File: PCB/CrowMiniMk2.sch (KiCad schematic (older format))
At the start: 21 parts

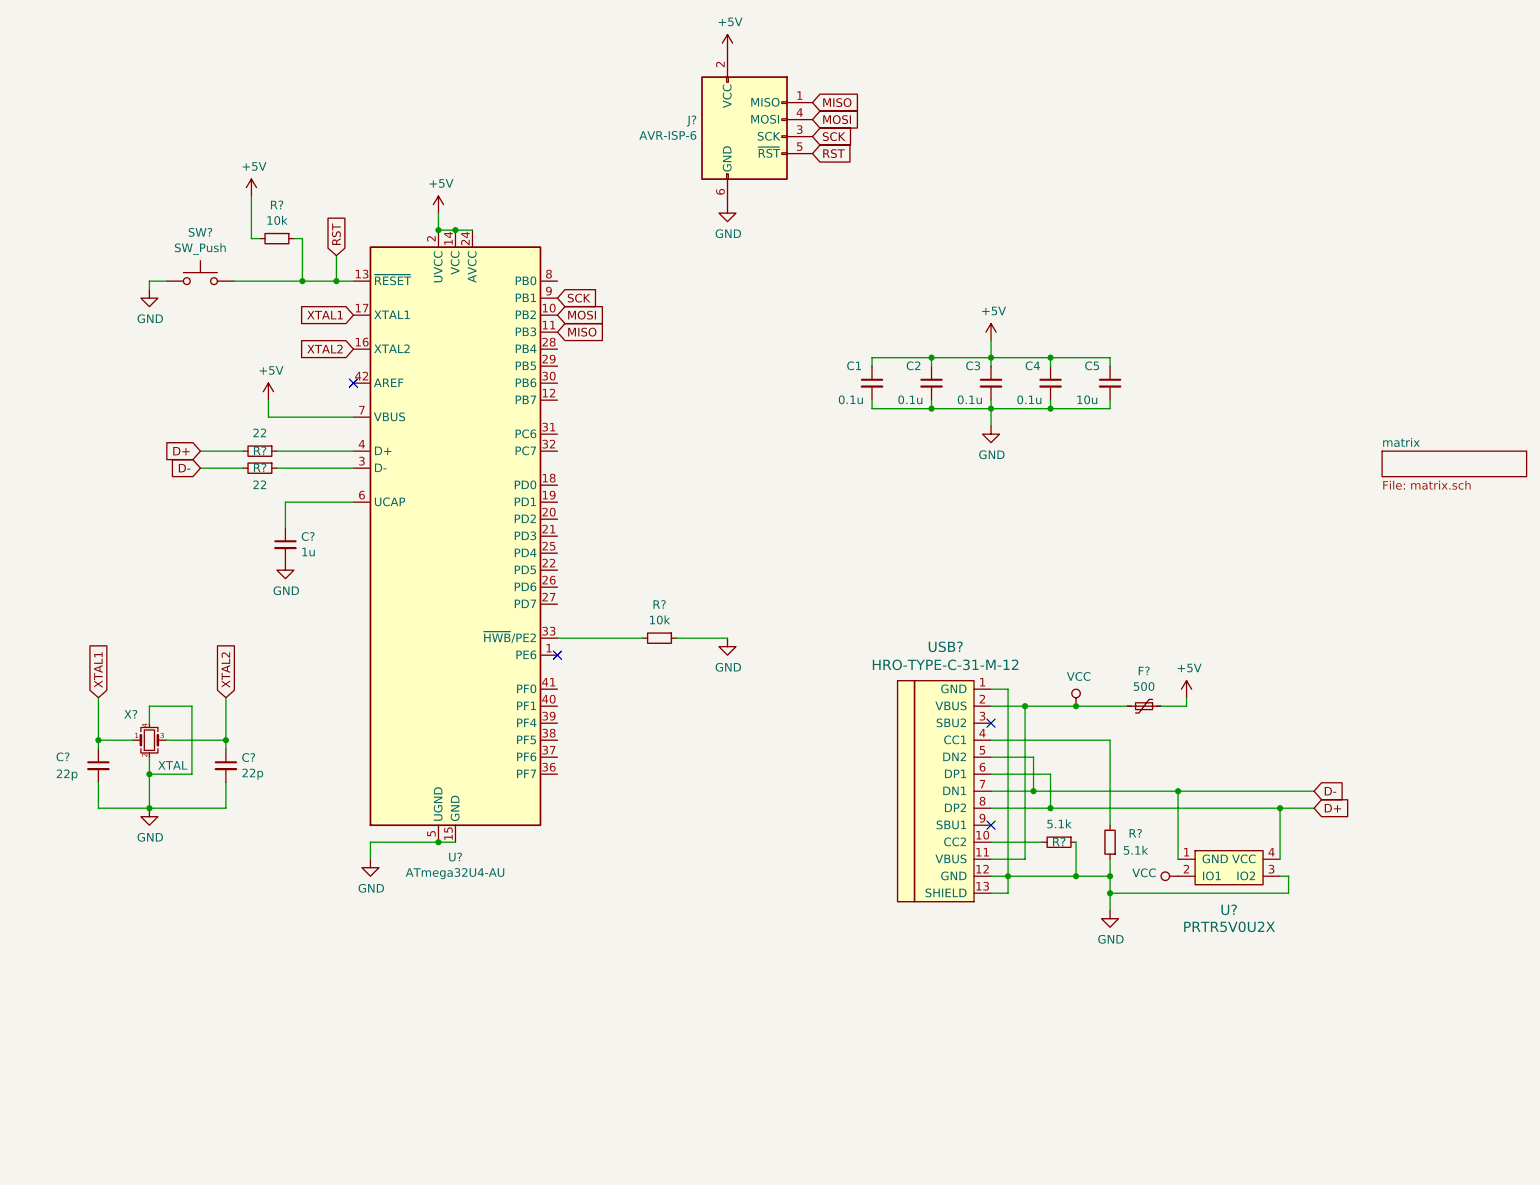
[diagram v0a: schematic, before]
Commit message: Sch Finish
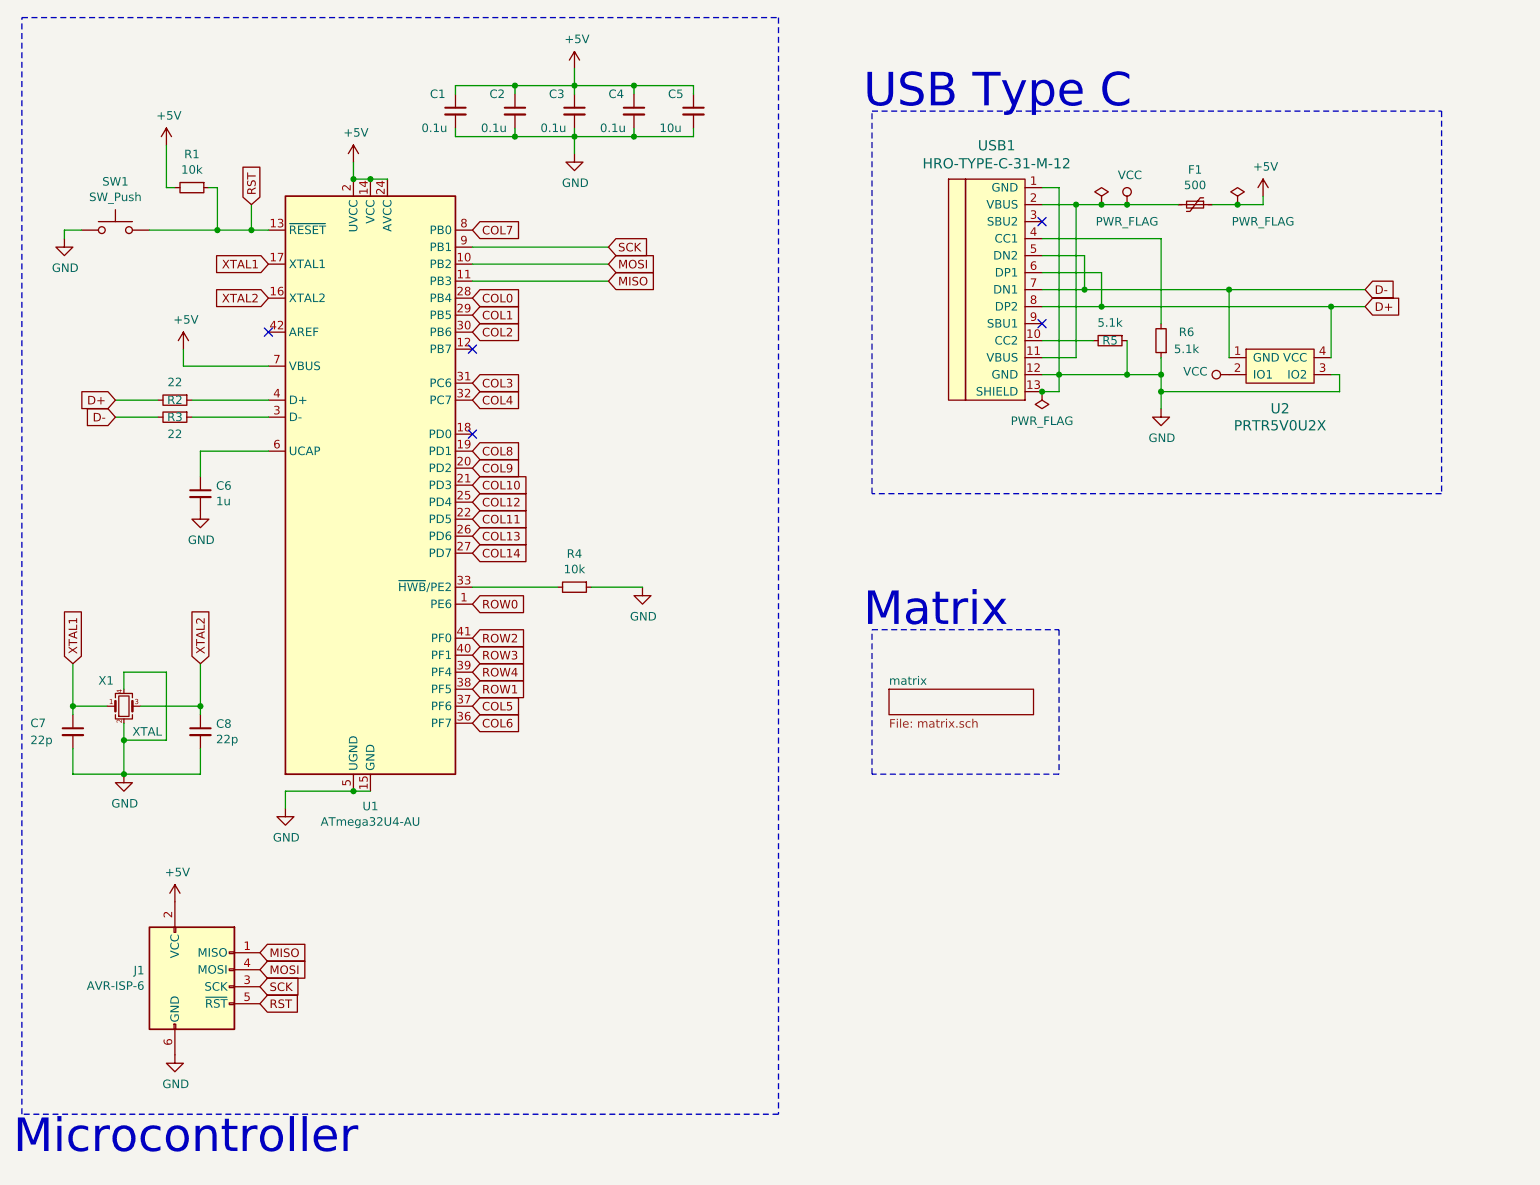
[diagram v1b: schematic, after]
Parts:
- C1, C2, C3, C4, C5: footprint (none) -> Capacitor_SMD:C_0805_2012Metric_Pad1.15x1.40mm_HandSolder
- C6, C7, C8: renamed from C?; footprint (none) -> Capacitor_SMD:C_0805_2012Metric_Pad1.15x1.40mm_HandSolder
- F1: renamed from F?; footprint (none) -> Fuse:Fuse_1206_3216Metric_Pad1.42x1.75mm_HandSolder
- J1: renamed from J?; footprint (none) -> random-keyboard-parts:Reset_Pretty-Mask
- R1, R2, R3, R4, R5, R6: renamed from R?; footprint (none) -> Resistor_SMD:R_0805_2012Metric_Pad1.15x1.40mm_HandSolder
- SW1: renamed from SW?; footprint (none) -> Button_Switch_SMD:SW_SPST_SKQG_WithStem
- U2: renamed from U?; footprint (none) -> random-keyboard-parts:SOT143B
- USB1: renamed from USB?; footprint (none) -> Type-C:HRO-TYPE-C-31-M-12-HandSoldering
- X1: renamed from X?; footprint (none) -> Crystal:Crystal_SMD_3225-4Pin_3.2x2.5mm_HandSoldering
- gave numbers to parts that had none: 1
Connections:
- net ROW0: now reaches U1.1 (PE6)
- net COL8: now reaches U1.19 (PD1)
- net COL9: now reaches U1.20 (PD2)
- net COL10: now reaches U1.21 (PD3)
- net COL11: now reaches U1.22 (PD5)
- net COL12: now reaches U1.25 (PD4)
- net COL13: now reaches U1.26 (PD6)
- net COL14: now reaches U1.27 (PD7)
- net COL0: now reaches U1.28 (PB4)
- net COL1: now reaches U1.29 (PB5)
- net COL2: now reaches U1.30 (PB6)
- net COL3: now reaches U1.31 (PC6)
- net COL4: now reaches U1.32 (PC7)
- net COL6: now reaches U1.36 (PF7)
- net COL5: now reaches U1.37 (PF6)
- net ROW1: now reaches U1.38 (PF5)
- net ROW4: now reaches U1.39 (PF4)
- net ROW3: now reaches U1.40 (PF1)
- net ROW2: now reaches U1.41 (PF0)
- net COL7: now reaches U1.8 (PB0)
- no-connect marks 4 -> 5
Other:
- note added: "Matrix"
- note added: "Microcontroller"
- note added: "USB Type C"
- moved on the sheet: C1, C2, C3, C4, C5, C6, C7, C8, F1, J1, R1, R2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
